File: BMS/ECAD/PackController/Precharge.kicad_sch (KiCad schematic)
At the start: 43 parts, among them K1101 KT12-1A-40L-THT, Q1101 DMP4065S-7, Q1102 IXTA08N100D2HV, Q1103 BC846, Q1104 IRLML0100TR, U1101 TCLT1004, U1102 TCLT1004, U1103 TEA1-0505HI, U1104 SN74LVC2G14DBV, U901 ADCMP393ARZ

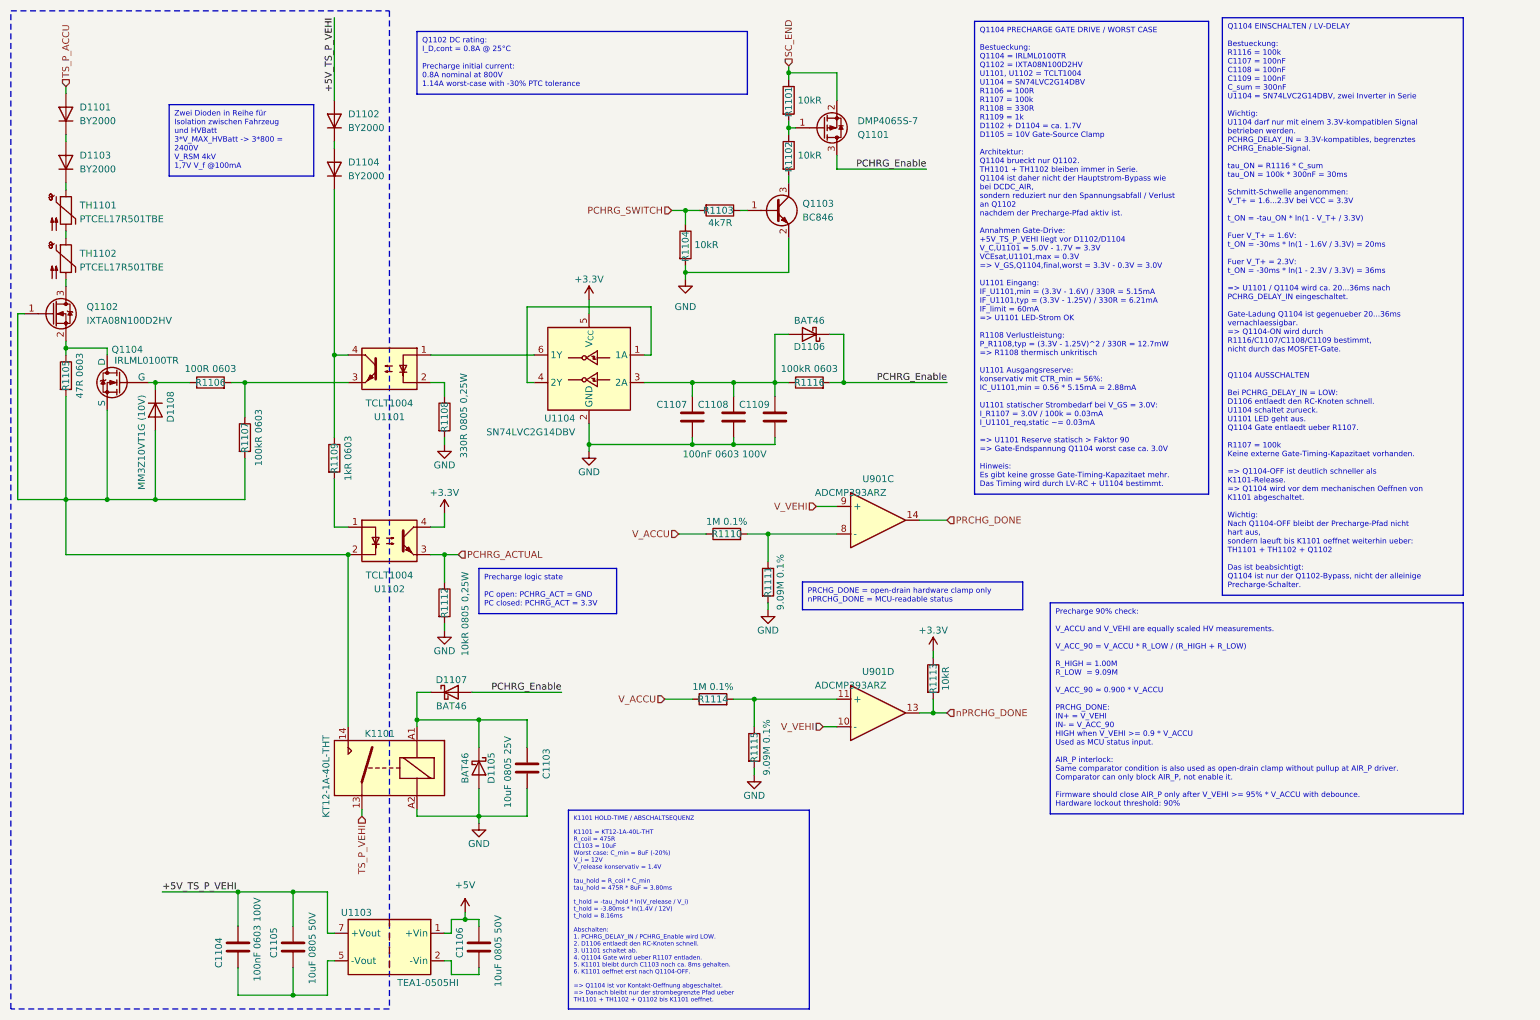
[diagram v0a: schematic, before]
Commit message: many fixes
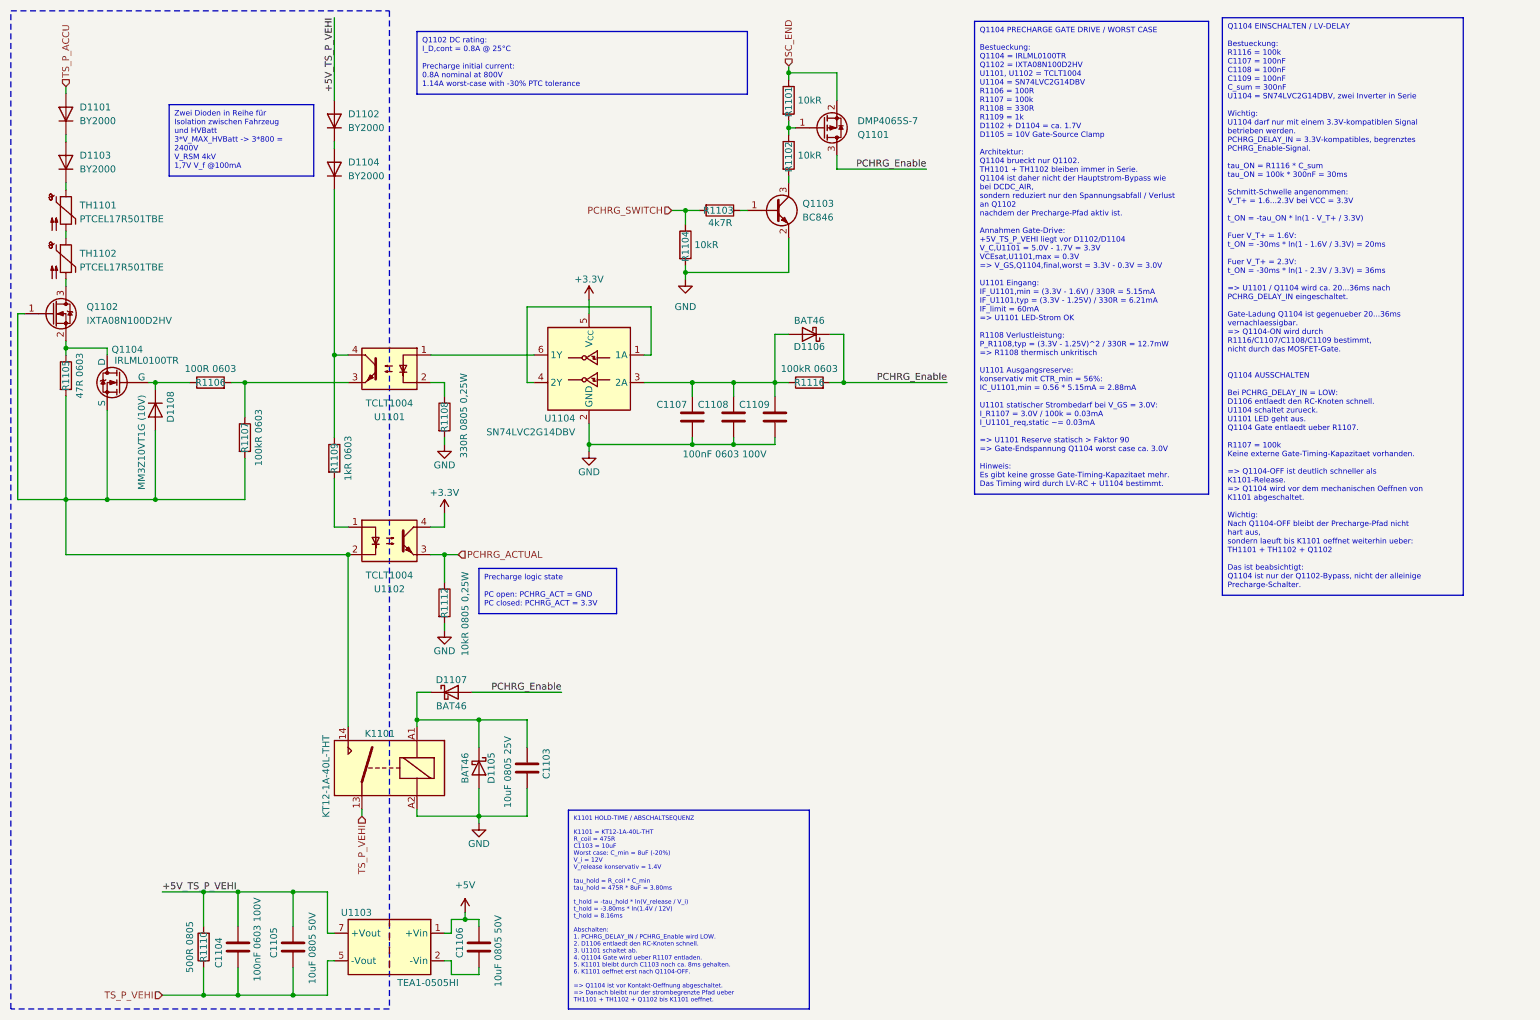
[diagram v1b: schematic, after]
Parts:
- removed R1111, R1115: 9.09M 0.1%, Resistor_SMD:R_0603_1608Metric_Pad0.98x0.95mm_HandSolder, symbol Device:R
- removed R1113: 10kR, Resistor_SMD:R_0603_1608Metric_Pad0.98x0.95mm_HandSolder, symbol Device:R
- removed R1114: 1M 0.1%, Resistor_SMD:R_0603_1608Metric_Pad0.98x0.95mm_HandSolder, symbol Device:R
- removed U901: ADCMP393ARZ, Package_SO:SOIC-14_3.9x8.7mm_P1.27mm, symbol EKartParts:ADCMP393ARUZ
- R1105: footprint Resistor_SMD:R_0603_1608Metric_Pad0.98x0.95mm_HandSolder -> Resistor_SMD:R_1206_3216Metric
- R1110: value 1M 0.1% -> 500R 0805; footprint Resistor_SMD:R_0603_1608Metric_Pad0.98x0.95mm_HandSolder -> Resistor_SMD:R_0805_2012Metric_Pad1.20x1.40mm_HandSolder
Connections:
- net V_ACCU is gone; now on net TS_P_VEHI: R1110.1
- net +5V_TS_P_VEHI: now also R1110.2
- net TS_P_VEHI: now also C1104.1, C1105.2, U1103.5 (-Vout)
